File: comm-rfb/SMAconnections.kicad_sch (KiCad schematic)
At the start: 4 parts, among them J6 Conn_Coaxial, J7 Conn_Coaxial, J8 Conn_Coaxial, J9 Conn_Coaxial

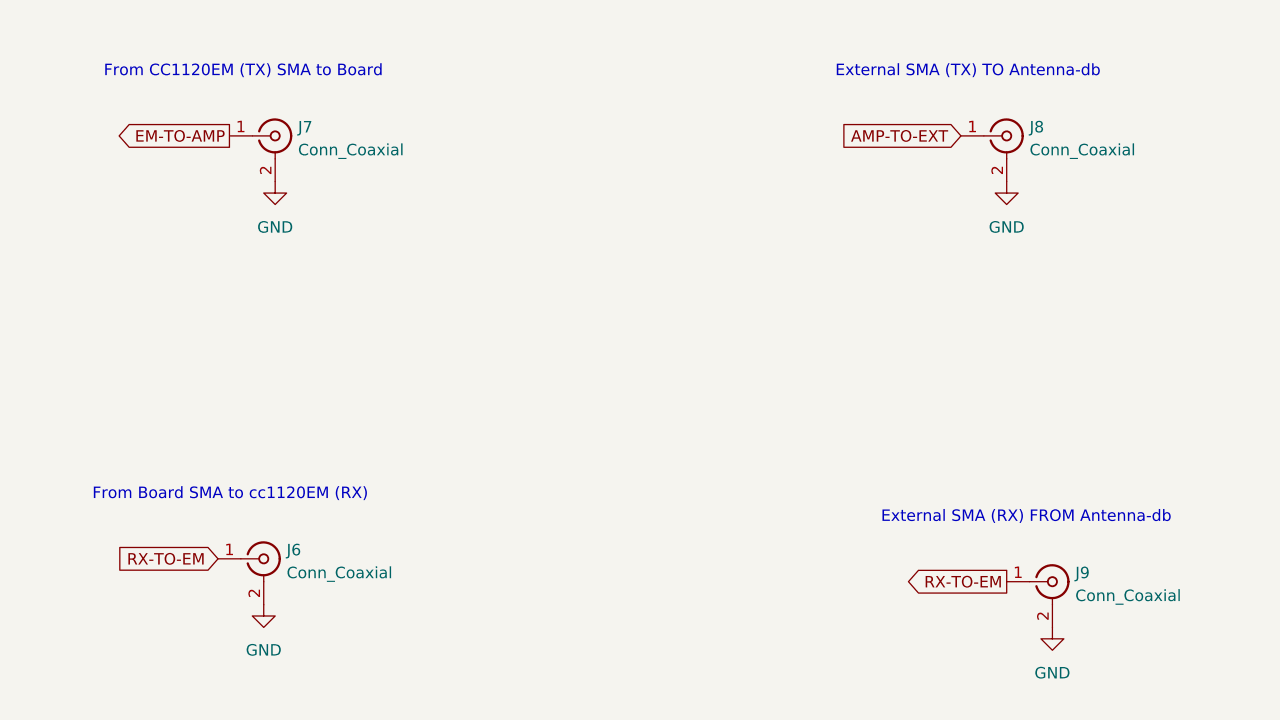
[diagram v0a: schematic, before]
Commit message: comm-rfb: reduce number of sheets in schematic
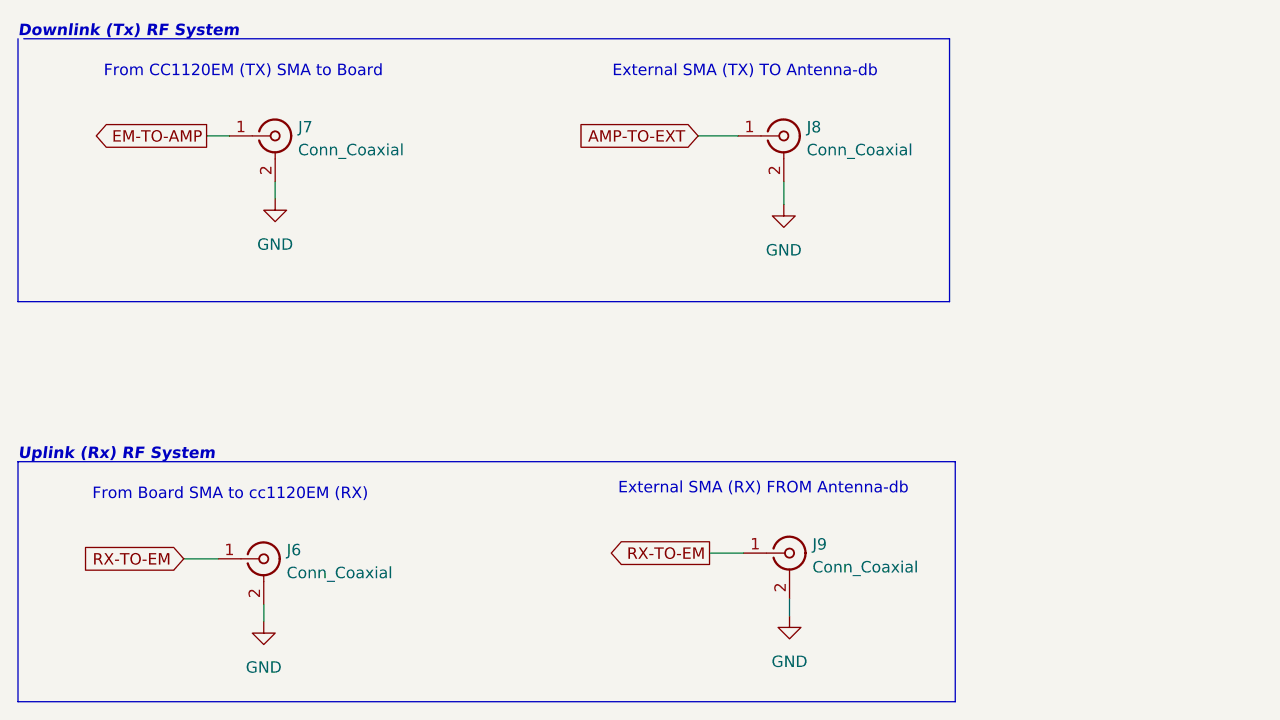
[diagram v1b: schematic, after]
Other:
- note added: "Downlink (Tx) RF System"
- note added: "Uplink (Rx) RF System"
- moved on the sheet: J8, J9
